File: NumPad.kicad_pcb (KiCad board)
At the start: 2 copper layers, 120.1 x 132.9 mm, 112 parts, among them J1 Micro_SD_Card_Det, J2 OLED1, J3 OLED2, J4 Conn_01x05_Female, SW1 SW_SPST, SW10 SW_SPST, SW11 SW_SPST, SW12 SW_SPST, SW13 SW_SPST, SW14 SW_SPST, SW15 SW_SPST, SW16 SW_SPST, SW17 SW_SPST, SW18 SW_SPST, SW19 SW_SPST, SW2 SW_SPST, SW20 SW_SPST, SW21 SW_SPST, SW22 SW_SPST, SW23 SW_SPST, SW24 SW_SPST, SW25 SW_BUTTONRESET, SW26 SW_BUTTON2, SW27 SW_BUTTON1, SW28 SW_BOOT0, SW29 Rotary_Encoder_Switch, SW3 SW_SPST, SW4 SW_SPST, SW5 SW_SPST, SW6 SW_SPST, SW7 SW_SPST, SW8 SW_SPST, SW9 SW_SPST, U1 LM117_TO3, U2 STM32F072C8Tx, U3 74AHCT1G08

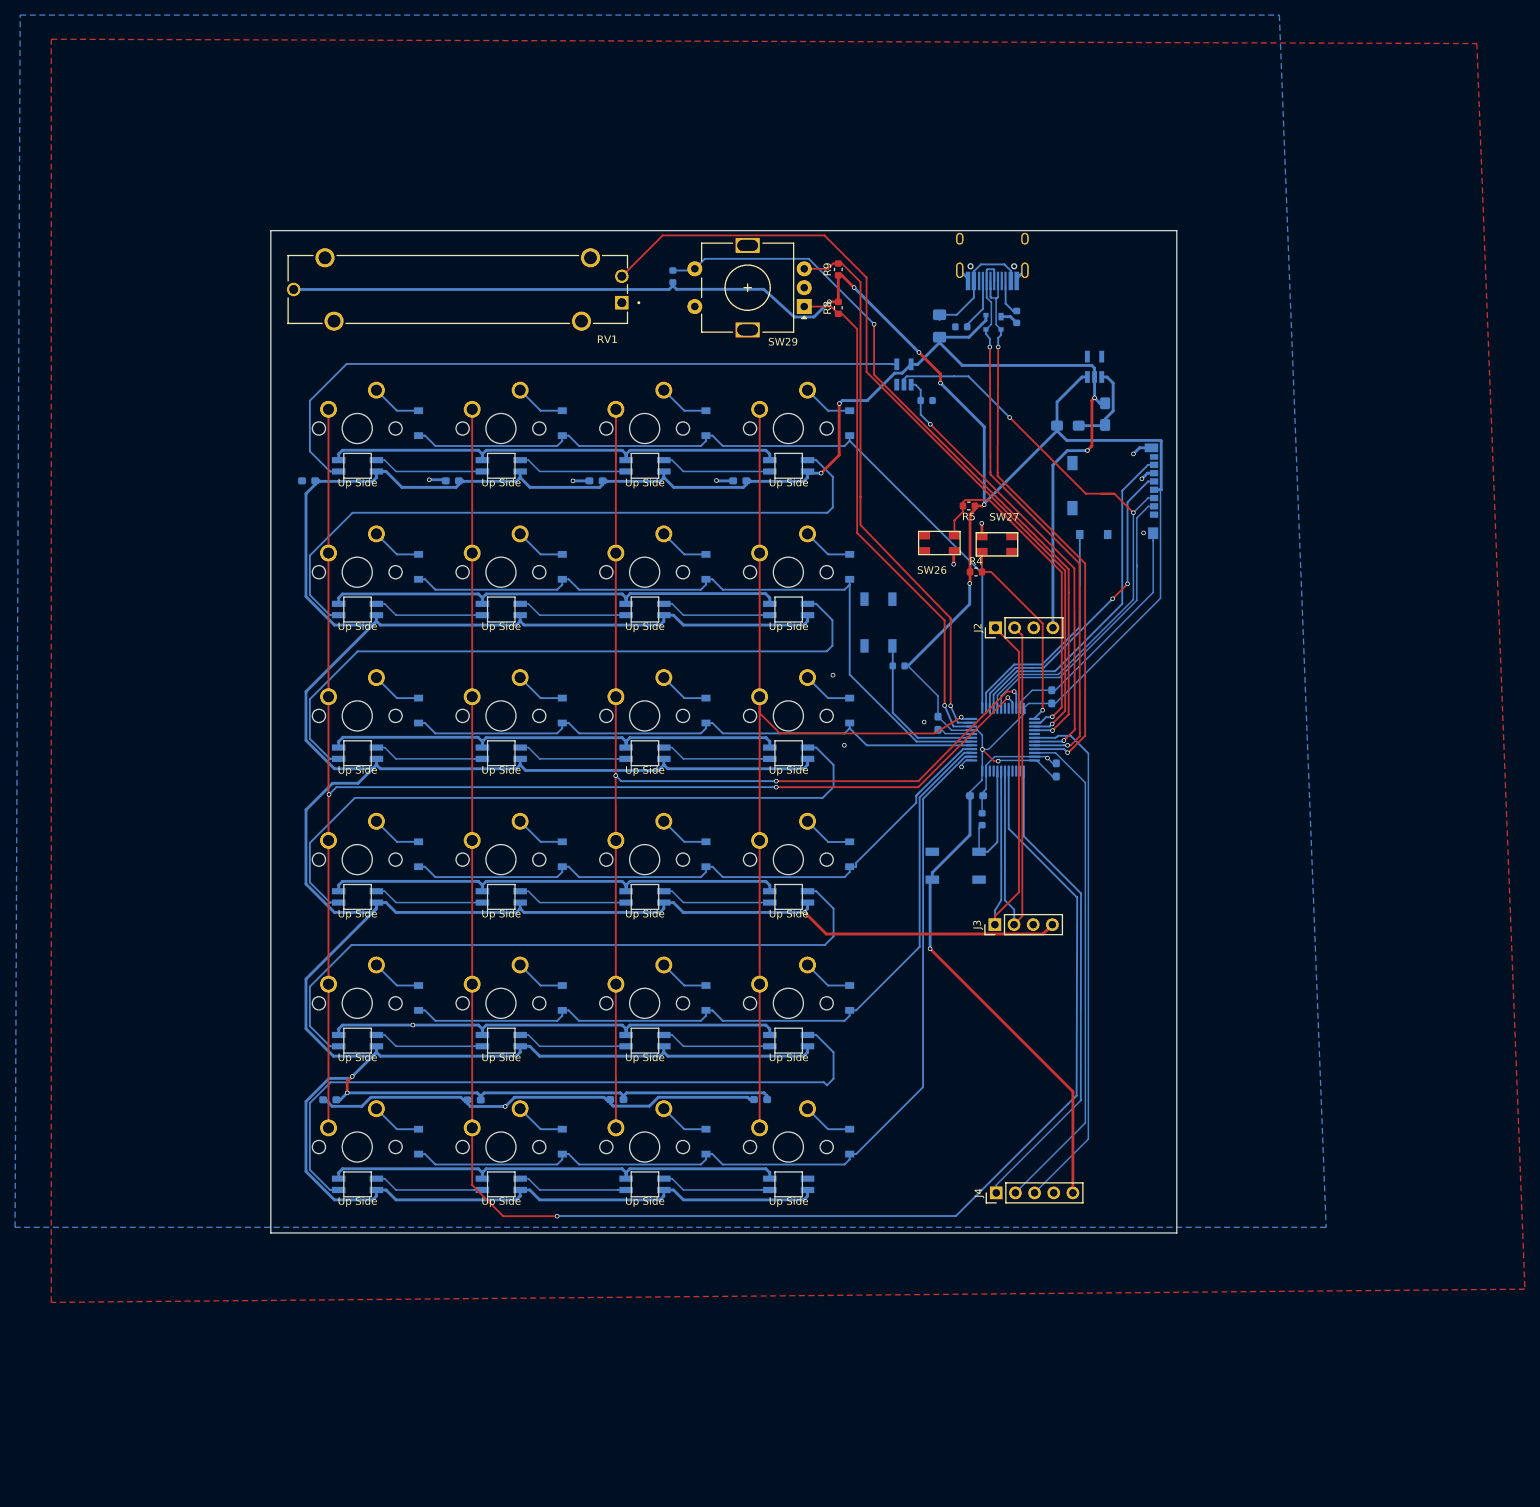
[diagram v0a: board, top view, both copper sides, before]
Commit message: update PCB
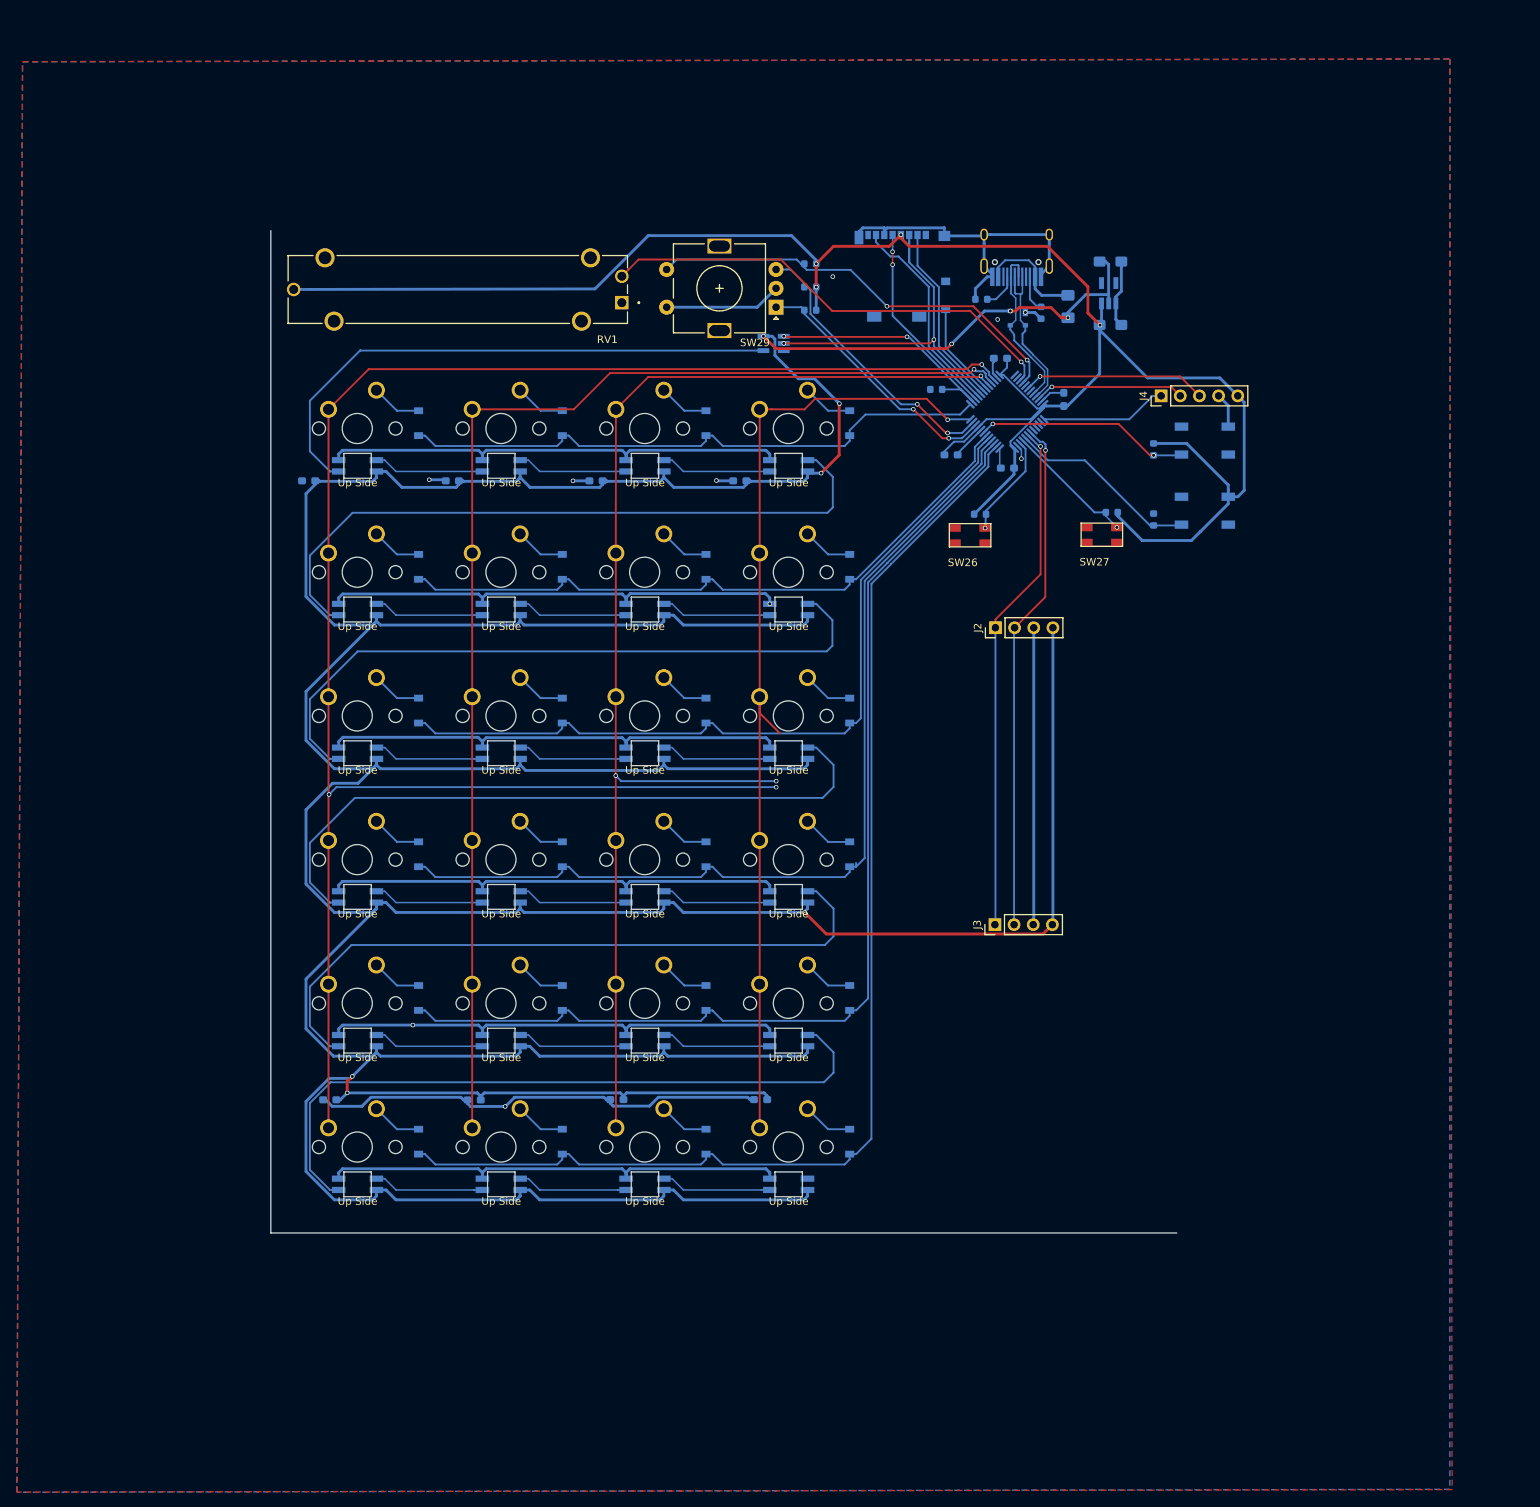
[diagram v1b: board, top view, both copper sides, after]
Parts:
- R4, R5, R8, R9: moved to B.Cu
- moved J4 107.9 mm to (137.9, 72.7)
- moved C6 58.1 mm to (116.6, 67.7), turned to 180 degrees
- moved SW28 57.5 mm to (143.7, 87.9), turned to 180 degrees
- moved SW25 49.5 mm to (143.7, 78.6), turned to 0 degrees
- moved R6 45.8 mm to (136.9, 89.1)
- moved R3 44.3 mm to (136.9, 79.8), turned to 270 degrees
- moved C5 44.0 mm to (110.1, 80.5), turned to 0 degrees
- moved U2 43.5 mm to (117.5, 74.8), turned to 45 degrees
- moved J1 39.9 mm to (103.6, 56.8), turned to 180 degrees
- moved C4 39.5 mm to (125.0, 73.2)
- moved C3 35.1 mm to (117.5, 82.3), turned to 180 degrees
- moved C1 20.2 mm to (131.2, 54.9), turned to 0 degrees
- moved R4 19.7 mm to (131.4, 88.2), turned to 180 degrees
- moved R10 18.3 mm to (91.4, 55.2), turned to 0 degrees
- moved U3 17.8 mm to (86.5, 65.8), turned to 180 degrees
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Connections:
- D49 pad 2: Net-(D49-Pad2) -> (no net)
- J1 pad 1: Net-(J1-Pad1) -> (no net)
- J1 pad 8: Net-(J1-Pad8) -> (no net)
- J1 pad 9: Net-(J1-Pad9) -> (no net)
- U2 pad 14: Detec -> LED_DATA_EN
- U2 pad 19: Net-(U2-Pad19) -> Detec
- U2 pad 20: Net-(U2-Pad20) -> col2
- U2 pad 21: col0 -> col1
- U2 pad 22: col2 -> col0
- U2 pad 25: BUT1 -> (no net)
- U2 pad 26: BUT2 -> (no net)
- U2 pad 29: Net-(U2-Pad29) -> (no net)
- U2 pad 31: LED_DATA_EN -> (no net)
- U2 pad 38: Net-(U2-Pad38) -> (no net)
- U2 pad 39: Net-(U2-Pad39) -> (no net)
- U2 pad 40: Net-(U2-Pad40) -> (no net)
- U2 pad 41: col1 -> (no net)
- U2 pad 45: Net-(U2-Pad45) -> BUT1
- U2 pad 46: Net-(U2-Pad46) -> BUT2
- USB1 pad 3: Net-(USB1-Pad3) -> (no net)
- USB1 pad 9: Net-(USB1-Pad9) -> (no net)
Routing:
- net +3V3: track 335.9 -> 262.9 mm, vias 9 -> 4
- net col1: track 238.1 -> 167.3 mm
- net USB_DP: track 76.0 -> 20.9 mm, vias 2 -> 0
- net col0: track 192.2 -> 246.8 mm
- net USB_DN: track 76.7 -> 22.7 mm, vias 2 -> 0
- net GND: track 528.2 -> 578.4 mm, vias 15 -> 11
- net POT_SLIDER: track 110.3 -> 62.3 mm
- net SYS_SWCLK: track 63.7 -> 16.8 mm
- net SYS_SWDIO: track 66.6 -> 19.9 mm, vias 0 -> 1
- net UART1_TX: track 69.4 -> 24.4 mm, vias 0 -> 1
- net row5: track 122.2 -> 164.3 mm
- net row4: track 103.7 -> 145.4 mm
- net row3: track 85.9 -> 127.1 mm
- net ENC_SWITCH: track 98.8 -> 57.7 mm
- net TIM2_CH2: track 74.0 -> 38.0 mm, vias 1 -> 2
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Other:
- outline, holes or cut-outs redrawn
- net class Default: clearance 0.2 -> 0.15
- net class power: clearance 0.2 -> 0.15
- rule trace_clearance: 0.2 -> 0.15
